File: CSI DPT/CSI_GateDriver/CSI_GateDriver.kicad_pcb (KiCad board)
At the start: 4 copper layers, 100 x 74.8 mm, 75 parts, among them J1 SSW-102-01-G-D, J2 Conn_02x08_Odd_Even, J3 SSW-102-01-G-D, Q3 DMP3099L, U1 UCC23513QDWYRQ1, U10 UCC23513QDWYRQ1, U11 MGJ2D121802SC, U12 LDK130-12_SOT23_SOT353, U2 MGJ2D121802SC, U3 MGJ2D121802SC, U4 LDK130-12_SOT23_SOT353, U5 NC7SZ125M5X, U6 NC7SZ125M5X, U7 ADM4168EBRUZ, U8 MGJ2D121802SC, U9 LT1086-ADJ

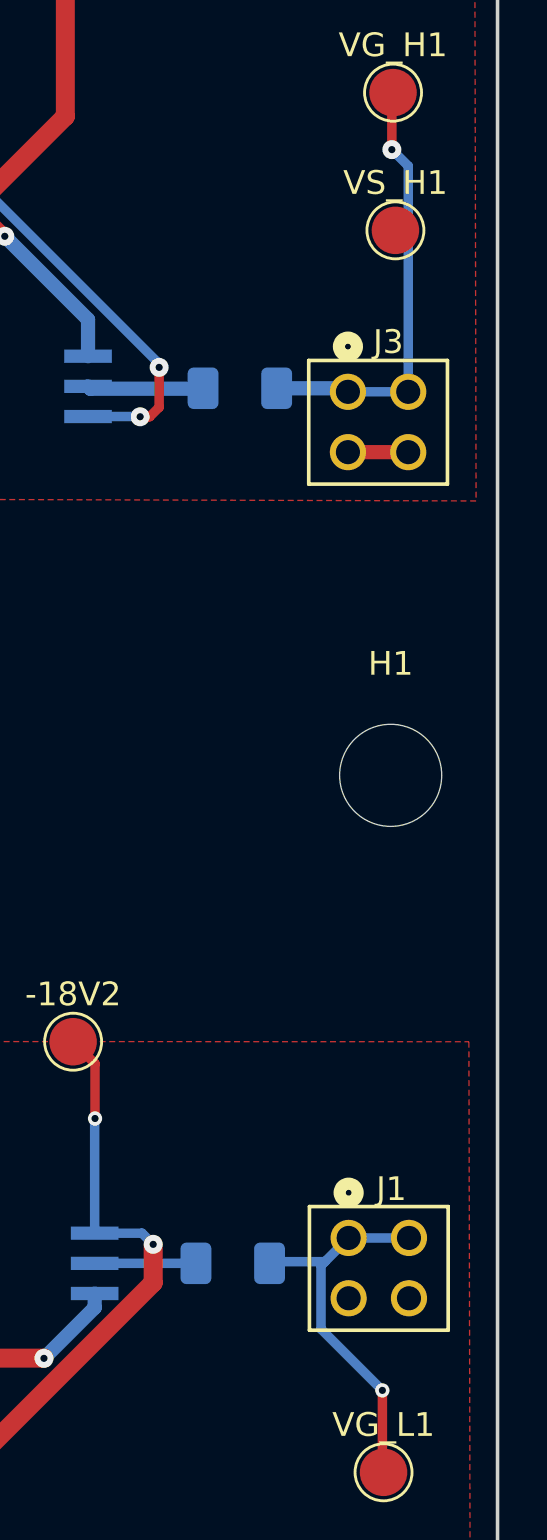
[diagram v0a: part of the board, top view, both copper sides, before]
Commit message: CSI Tester V1 Completed
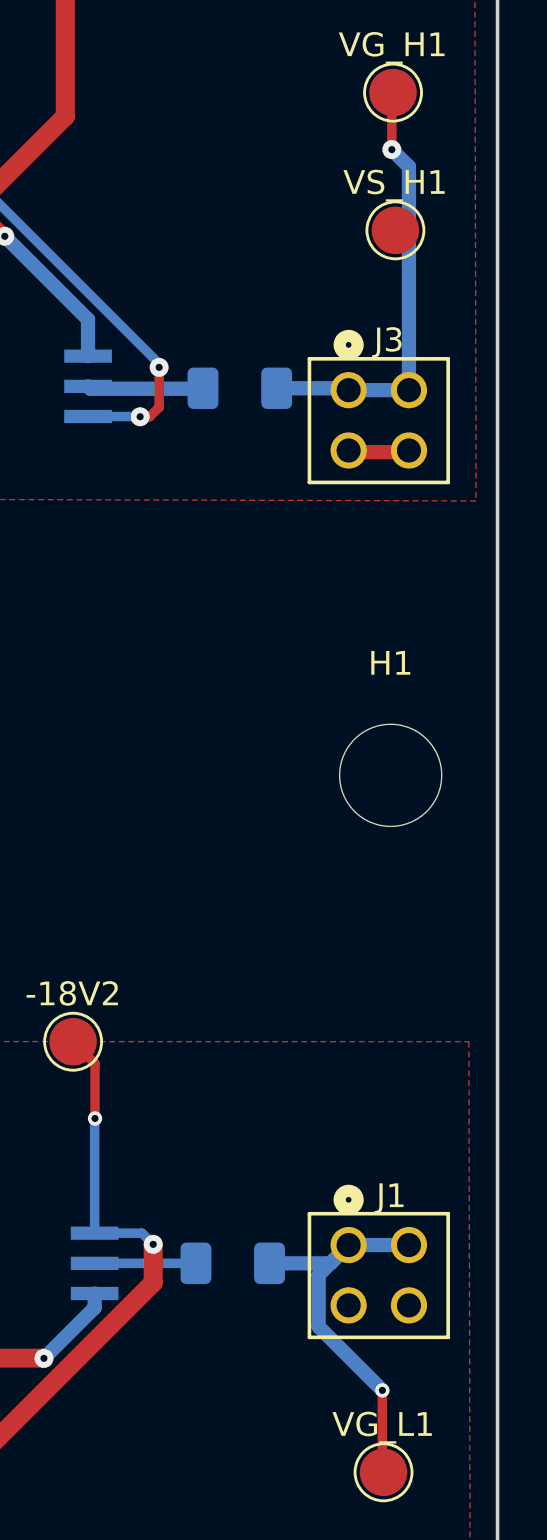
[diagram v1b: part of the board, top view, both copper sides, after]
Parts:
- moved J1 0.30 mm to (161.0, 119.9)
- moved J3 0.08 mm to (161.0, 83.9)
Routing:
- net /Gate_Driver/VGATE_L: track 16.3 -> 17.4 mm
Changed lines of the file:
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@@
 	(footprint "Gate_Driver:CON4_2X2_TU_SSQ"
 		(layer "F.Cu")
-		(at 160.97 83.97 180)
+		(at 161 83.9 180)
 		(tags "SSW-102-01-G-D ")
 		(property "Reference" "J3"
@@
 	(footprint "Gate_Driver:CON4_2X2_TU_SSQ"
 		(layer "F.Cu")
-		(at 161 119.6 180)
+		(at 161 119.9 180)
 		(tags "SSW-102-01-G-D ")
 		(property "Reference" "J1"
@@
 	(segment
 		(start 156.7 82.55)
-		(end 159.55 82.55)
+		(end 159.65 82.55)
 		(width 0.6)
 		(layer "B.Cu")
@@
 	)
 	(segment
-		(start 162.24 73.19)
-		(end 161.55 72.5)
-		(width 0.4)
-		(layer "B.Cu")
-		(net 9)
-	)
-	(segment
-		(start 159.55 82.55)
-		(end 159.7 82.7)
+		(start 162.27 82.63)
+		(end 162.27 73.22)
 		(width 0.6)
 		(layer "B.Cu")
@@
 	)
 	(segment
-		(start 159.7 82.7)
-		(end 162.24 82.7)
-		(width 0.4)
+		(start 159.65 82.55)
+		(end 159.73 82.63)
+		(width 0.6)
 		(layer "B.Cu")
 		(net 9)
 	)
 	(segment
-		(start 162.24 82.7)
-		(end 162.24 73.19)
-		(width 0.4)
+		(start 162.27 73.22)
+		(end 161.55 72.5)
+		(width 0.6)
 		(layer "B.Cu")
 		(net 9)
 	)
 	(segment
-		(start 159.6 82.6)
-		(end 159.7 82.7)
-		(width 0.4)
+		(start 159.73 82.63)
+		(end 162.27 82.63)
+		(width 0.6)
 		(layer "B.Cu")
 		(net 9)
@@
 	)
 	(segment
-		(start 158.567 119.493)
-		(end 158.567 122.167)
-		(width 0.4)
-		(layer "B.Cu")
-		(net 44)
-	)
-	(segment
-		(start 158.73 119.33)
-		(end 158.567 119.493)
-		(width 0.4)
+		(start 159.73 118.63)
+		(end 158.467 119.893)
+		(width 0.6)
 		(layer "B.Cu")
 		(net 44)
 	)
 	(segment
-		(start 158.73 119.33)
-		(end 159.73 118.33)
-		(width 0.4)
+		(start 159.73 118.63)
+		(end 162.27 118.63)
+		(width 0.6)
 		(layer "B.Cu")
 		(net 44)
 	)
 	(segment
-		(start 159.73 118.33)
-		(end 162.27 118.33)
-		(width 0.4)
+		(start 156.4 119.4)
+		(end 158.96 119.4)
+		(width 0.6)
 		(layer "B.Cu")
 		(net 44)
 	)
 	(segment
-		(start 156.4 119.4)
-		(end 156.47 119.33)
-		(width 0.4)
+		(start 158.467 119.893)
+		(end 158.467 122.067)
+		(width 0.6)
 		(layer "B.Cu")
 		(net 44)
 	)
 	(segment
-		(start 156.47 119.33)
-		(end 158.73 119.33)
-		(width 0.4)
+		(start 158.96 119.4)
+		(end 159.73 118.63)
+		(width 0.6)
 		(layer "B.Cu")
 		(net 44)
 	)
 	(segment
-		(start 158.567 122.167)
+		(start 158.467 122.067)
 		(end 161.15 124.75)
-		(width 0.4)
+		(width 0.6)
 		(layer "B.Cu")
 		(net 44)
